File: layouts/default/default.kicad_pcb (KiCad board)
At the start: 2 copper layers, 41.9 x 34.7 mm, 37 parts

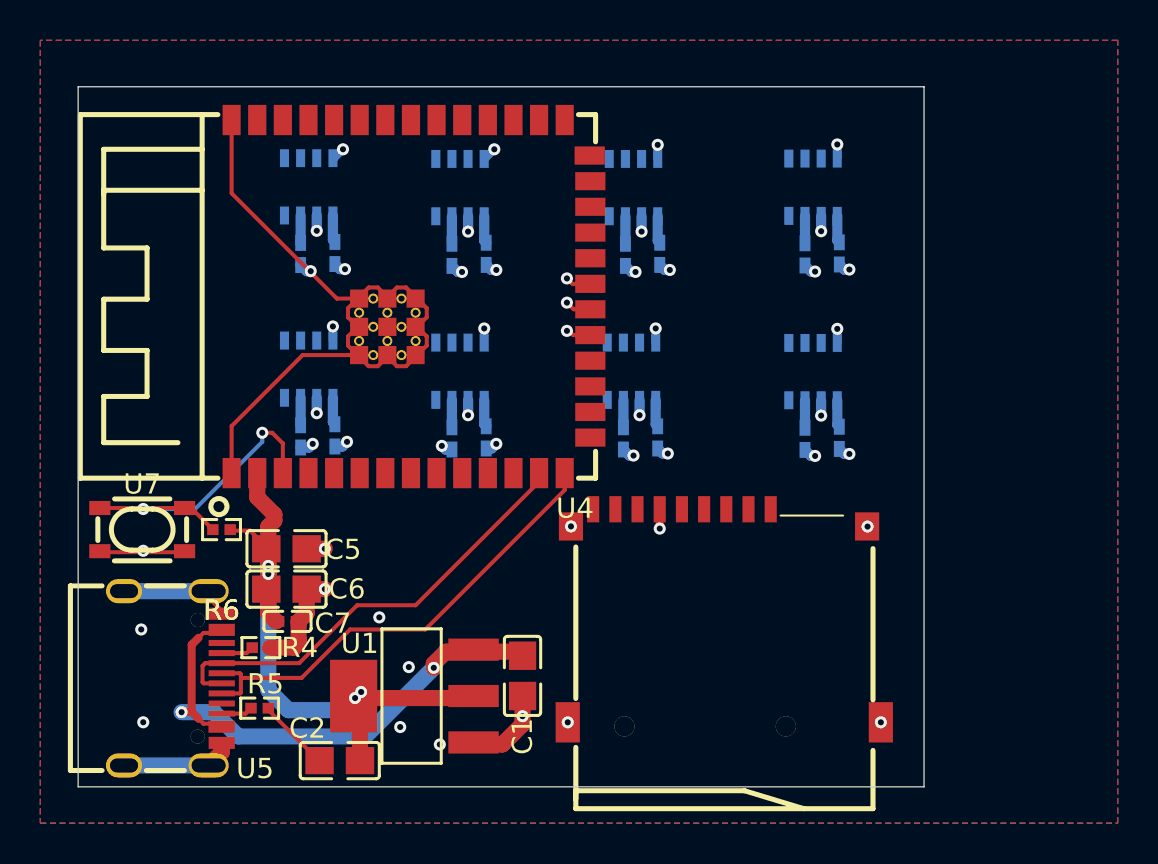
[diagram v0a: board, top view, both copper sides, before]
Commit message: doneish
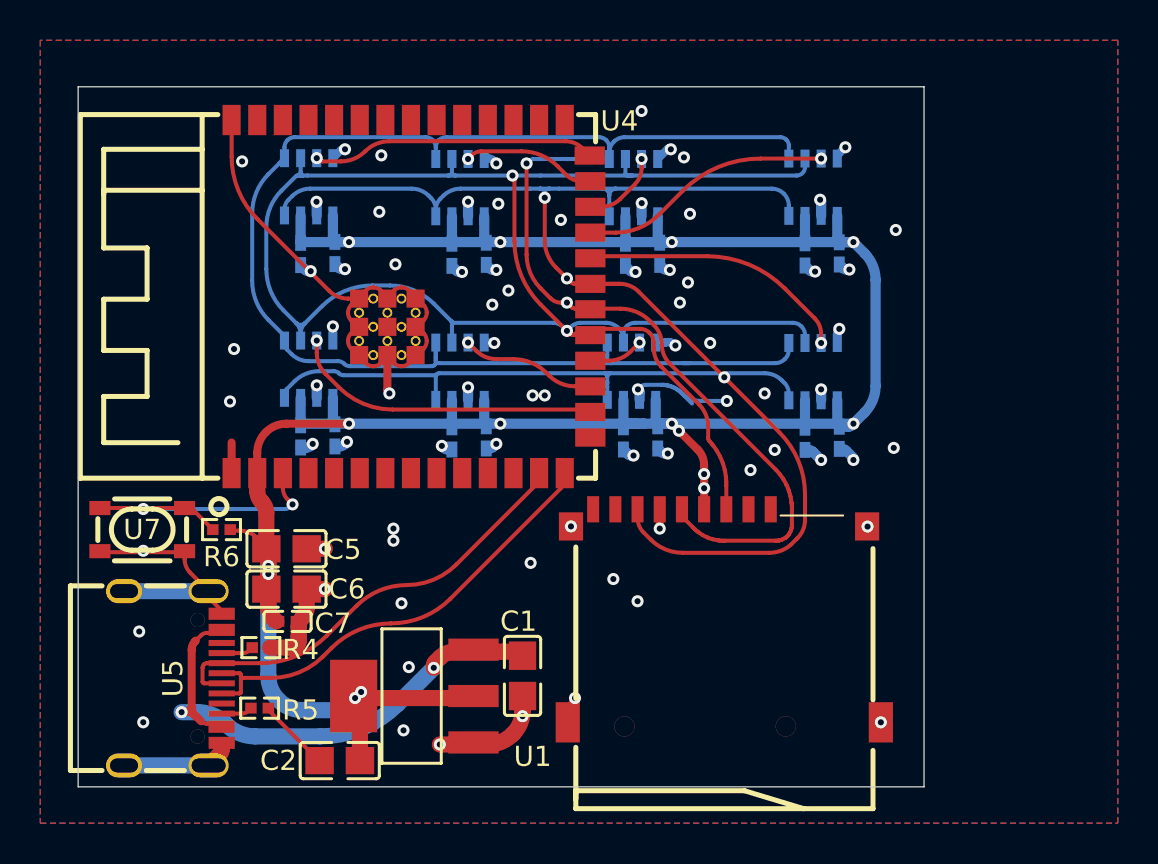
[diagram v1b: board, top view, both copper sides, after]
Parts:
- R4, R5: value 4.7kΩ ±1% 62.5mW -> 5.1kΩ ±1% 62.5mW
- R6: value 10kΩ ±1% 62.5mW -> 10kΩ ±5% 62.5mW
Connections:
- net B8 renamed SUB2
- net SUB1 renamed A8
- U10 pad 2: noses[4]-CSB -> CSB-4
- U11 pad 2: noses[5]-CSB -> line
- U12 pad 2: noses[6]-CSB -> CSB-3
- U13 pad 2: noses[7]-CSB -> CSB-6
- U2 pad 2: noses[0]-CSB -> CSB-5
- U3 pad 2: noses[1]-CSB -> CSB-1
- U4 pad 16: io46 -> CSB-6
- U4 pad 17: io9 -> CSB-3
- U4 pad 22: io14 -> CSB-4
- U4 pad 23: io21 -> CSB
- U4 pad 24: io47 -> CSB-2
- U4 pad 25: io48 -> CSB-1
- U4 pad 26: io45 -> CSB-5
- U8 pad 2: noses[2]-CSB -> CSB-2
- U9 pad 2: noses[3]-CSB -> CSB
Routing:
- net SCK: track 1.44 -> 105.6 mm, vias 1 -> 2
- net SDO: track 1.27 -> 96.2 mm, vias 1 -> 3
- net SDI: track 1.25 -> 92.6 mm, vias 1 -> 2
- net hv: track 54.1 -> 135.2 mm, vias 4 -> 15
- net CSB-6: track 0.00 -> 15.5 mm, vias 0 -> 1
- net CSB-5: track 0.00 -> 14.1 mm, vias 0 -> 1
- net CSB-4: track 0.00 -> 13.5 mm, vias 0 -> 1
- net CSB: track 0.00 -> 12.6 mm, vias 0 -> 1
- net CSB-3: track 0.00 -> 6.69 mm, vias 0 -> 1
- net CSB-1: track 0.00 -> 6.63 mm, vias 0 -> 1
- net gnd: track 89.0 -> 93.6 mm, vias 34 -> 75
- net CSB-2: track 0.00 -> 3.94 mm, vias 0 -> 1
- net line: track 0.00 -> 2.74 mm, vias 0 -> 1
- net input: track 19.0 -> 17.8 mm
- net io20: track 23.6 -> 23.0 mm
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- added copper zone on B.Cu, net gnd
- added copper zone on F.Cu, net gnd
- removed copper zone on B.Cu, net (none)
- removed copper zone on F.Cu, net (none)

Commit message: meow
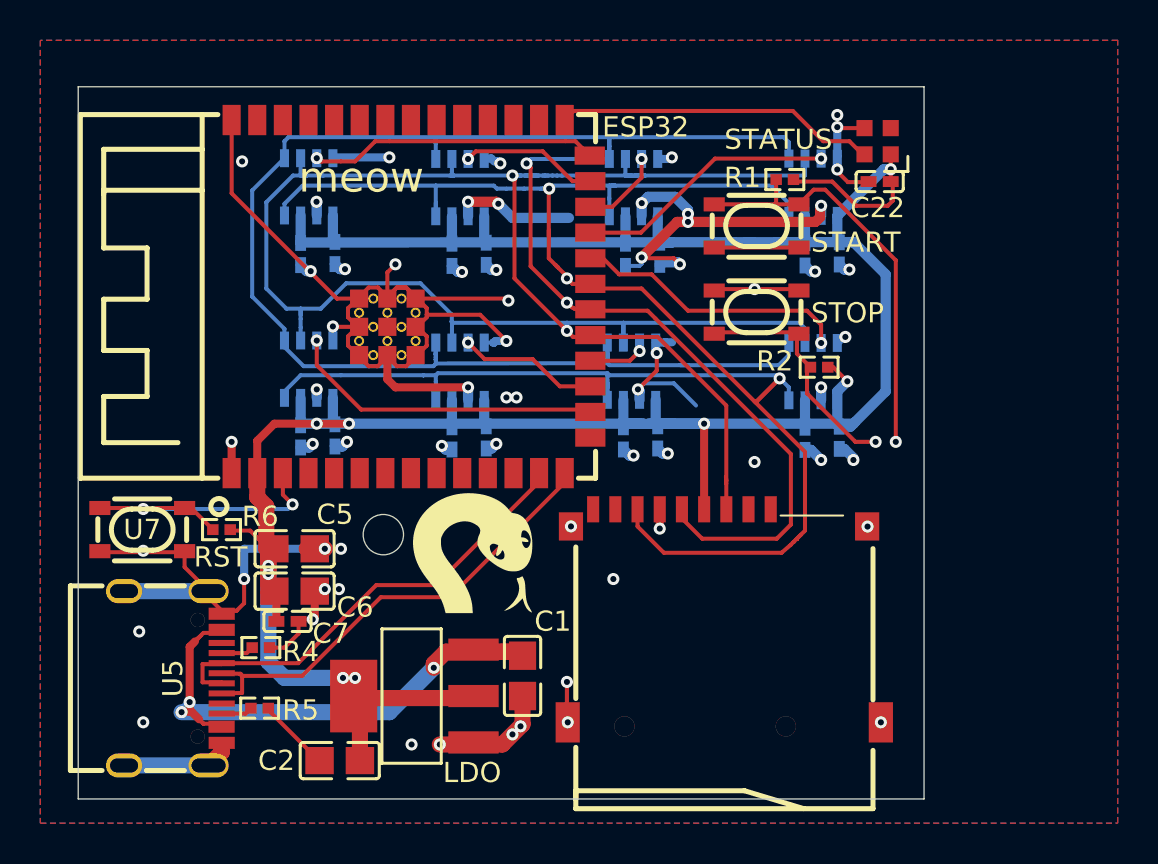
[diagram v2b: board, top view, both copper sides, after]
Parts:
- added C22: 100nF ±10% 16V X7R, atopile:C0402-b3ef17, F.Cu at (109.8, 65.0)
- added R1: 10kΩ ±1% 62.5mW, atopile:R0402-56259e, F.Cu at (105.1, 64.9)
- added R2: 10kΩ ±1% 62.5mW, atopile:R0402-56259e, F.Cu at (106.8, 74.2)
- added U14: , lib:LED-SMD_4P-L2.0-W2.0-BR, F.Cu at (109.7, 63.0)
- added U15: , lib:KEY-SMD_4P-L4.2-W3.2-P2.20-LS4.6, F.Cu at (103.7, 67.2)
- added U16: , lib:KEY-SMD_4P-L4.2-W3.2-P2.20-LS4.6, F.Cu at (103.7, 71.5)
- R6: value 10kΩ ±5% 62.5mW -> 10kΩ ±1% 62.5mW
- moved C6 0.41 mm to (80.8, 85.3)
- moved C5 0.40 mm to (80.8, 83.2)
- renumbered U4 to ESP32, U1 to LDO, U2 to SEN1, U3 to SEN2, U9 to SEN4, U13 to SEN5, U12 to SEN6, U11 to SEN7, U10 to SEN8
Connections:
- net A5 renamed CC1
- net A8 renamed SUB1
- net CC2 renamed B5
- net SUB2 renamed B8
- net input renamed input-1
- net io16 renamed line-2
- C1 pad 1: hv-1 -> hv
- C10 pad 1: hv -> hv-1
- C11 pad 1: hv -> hv-1
- C12 pad 1: hv -> hv-1
- C13 pad 1: hv -> hv-1
- C14 pad 1: hv -> hv-1
- C15 pad 1: hv -> hv-1
- C16 pad 1: hv -> hv-1
- C17 pad 1: hv -> hv-1
- C18 pad 1: hv -> hv-1
- C19 pad 1: hv -> hv-1
- C2 pad 1: hv -> hv-1
- C20 pad 1: hv -> hv-1
- C21 pad 1: hv -> hv-1
- C3 pad 1: hv -> hv-1
- C4 pad 1: hv -> hv-1
- C5 pad 1: hv -> hv-1
- C6 pad 1: hv -> hv-1
- C7 pad 1: hv -> hv-1
- C8 pad 1: hv -> hv-1
- C9 pad 1: hv -> hv-1
- ESP32 pad 16: CSB-6 -> CSB-3
- ESP32 pad 17: CSB-3 -> CSB-5
- ESP32 pad 18: line -> line-1
- ESP32 pad 2: hv -> hv-1
- ESP32 pad 23: CSB -> CSB-6
- ESP32 pad 24: CSB-2 -> CSB-1
- ESP32 pad 25: CSB-1 -> CSB
- ESP32 pad 26: CSB-5 -> CSB-2
- ESP32 pad 27: io0 -> DIN
- ESP32 pad 8: io15 -> line
- LDO pad 2: hv -> hv-1
- LDO pad 3: hv-1 -> hv
- LDO pad 4: hv -> hv-1
- R6 pad 1: hv -> hv-1
- SEN1 pad 2: CSB-5 -> CSB-2
- SEN1 pad 6: hv -> hv-1
- SEN1 pad 8: hv -> hv-1
- SEN2 pad 2: CSB-1 -> CSB
- SEN2 pad 6: hv -> hv-1
- SEN2 pad 8: hv -> hv-1
- SEN4 pad 2: CSB -> CSB-6
- SEN4 pad 6: hv -> hv-1
- SEN4 pad 8: hv -> hv-1
- SEN5 pad 2: CSB-6 -> CSB-3
- SEN5 pad 6: hv -> hv-1
- SEN5 pad 8: hv -> hv-1
- SEN6 pad 2: CSB-3 -> CSB-5
- SEN6 pad 6: hv -> hv-1
- SEN6 pad 8: hv -> hv-1
- SEN7 pad 2: line -> line-1
- SEN7 pad 6: hv -> hv-1
- SEN7 pad 8: hv -> hv-1
- SEN8 pad 6: hv -> hv-1
- SEN8 pad 8: hv -> hv-1
- U5 pad A4: hv-1 -> hv
- U5 pad A9: hv-1 -> hv
- U5 pad B4: hv-1 -> hv
- U5 pad B9: hv-1 -> hv
- U6 pad 4: hv -> hv-1
- U8 pad 2: CSB-2 -> CSB-1
- U8 pad 6: hv -> hv-1
- U8 pad 8: hv -> hv-1
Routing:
- net hv-1: track 27.0 -> 151.9 mm, vias 2 -> 9
- net hv: track 135.2 -> 26.8 mm, vias 15 -> 3
- net gnd: track 93.6 -> 158.0 mm, vias 75 -> 65
- net input-2: track 0.00 -> 20.9 mm, vias 0 -> 1
- net DIN: track 0.00 -> 15.9 mm
- net input: track 0.00 -> 11.9 mm, vias 0 -> 1
- net CSB-2: track 3.94 -> 14.3 mm
- net CSB-3: track 6.69 -> 15.7 mm
- net CSB-5: track 14.1 -> 6.96 mm
- net CSB: track 12.6 -> 6.83 mm
- net SDO: track 96.2 -> 100.3 mm
- net line: track 2.74 -> 0.00 mm, vias 1 -> 0
- net line-1: track 0.00 -> 2.64 mm, vias 0 -> 1
- net CSB-1: track 6.63 -> 4.06 mm
- net CSB-6: track 15.5 -> 13.0 mm
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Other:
- board size 41.9 x 34.7 mm -> 41.9 x 35.3 mm
- board text added: "RST"
- board text added: "START"
- board text added: "STATUS"
- board text added: "STOP"
- board text added: "lucy m 05/25"
- board text added: "meow"
- board text added: "non human scent"
- board text removed: "04/25/25 NonHumanScent"
- board text removed: "eigenlucy/nonhumanscent"
